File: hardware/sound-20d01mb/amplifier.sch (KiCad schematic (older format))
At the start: 30 parts

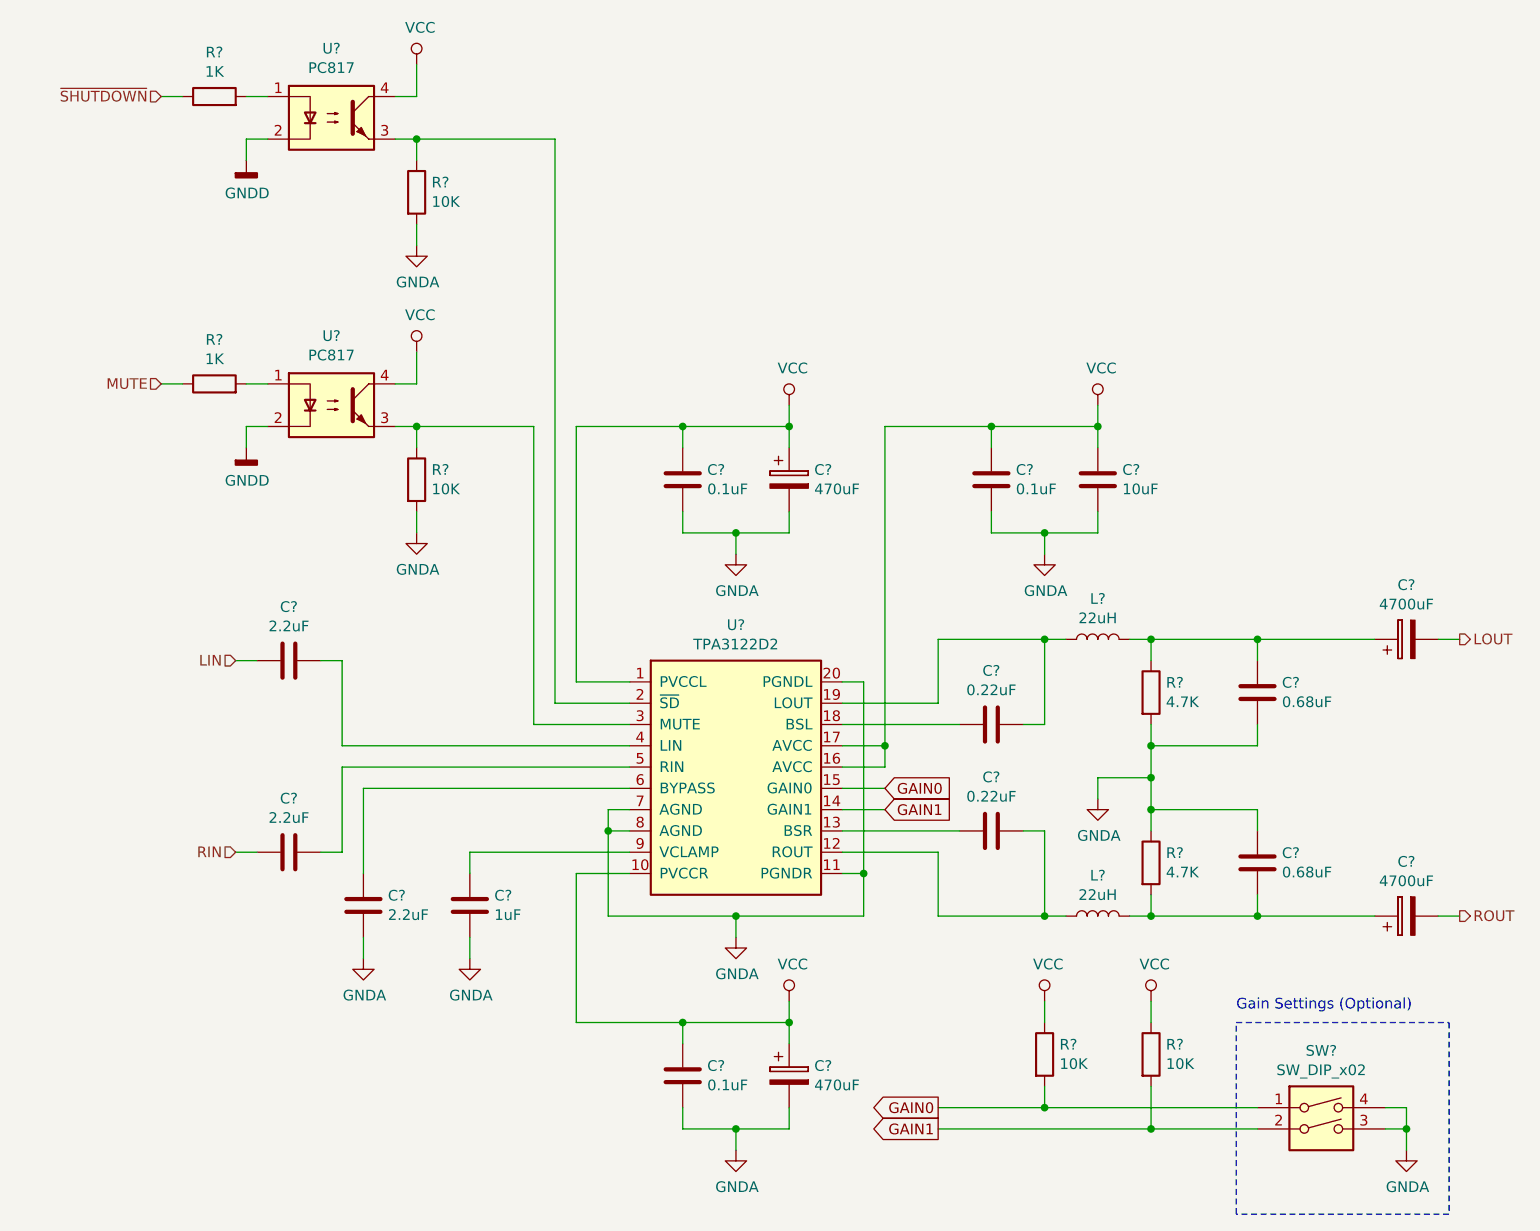
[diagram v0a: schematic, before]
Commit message: Added OSC
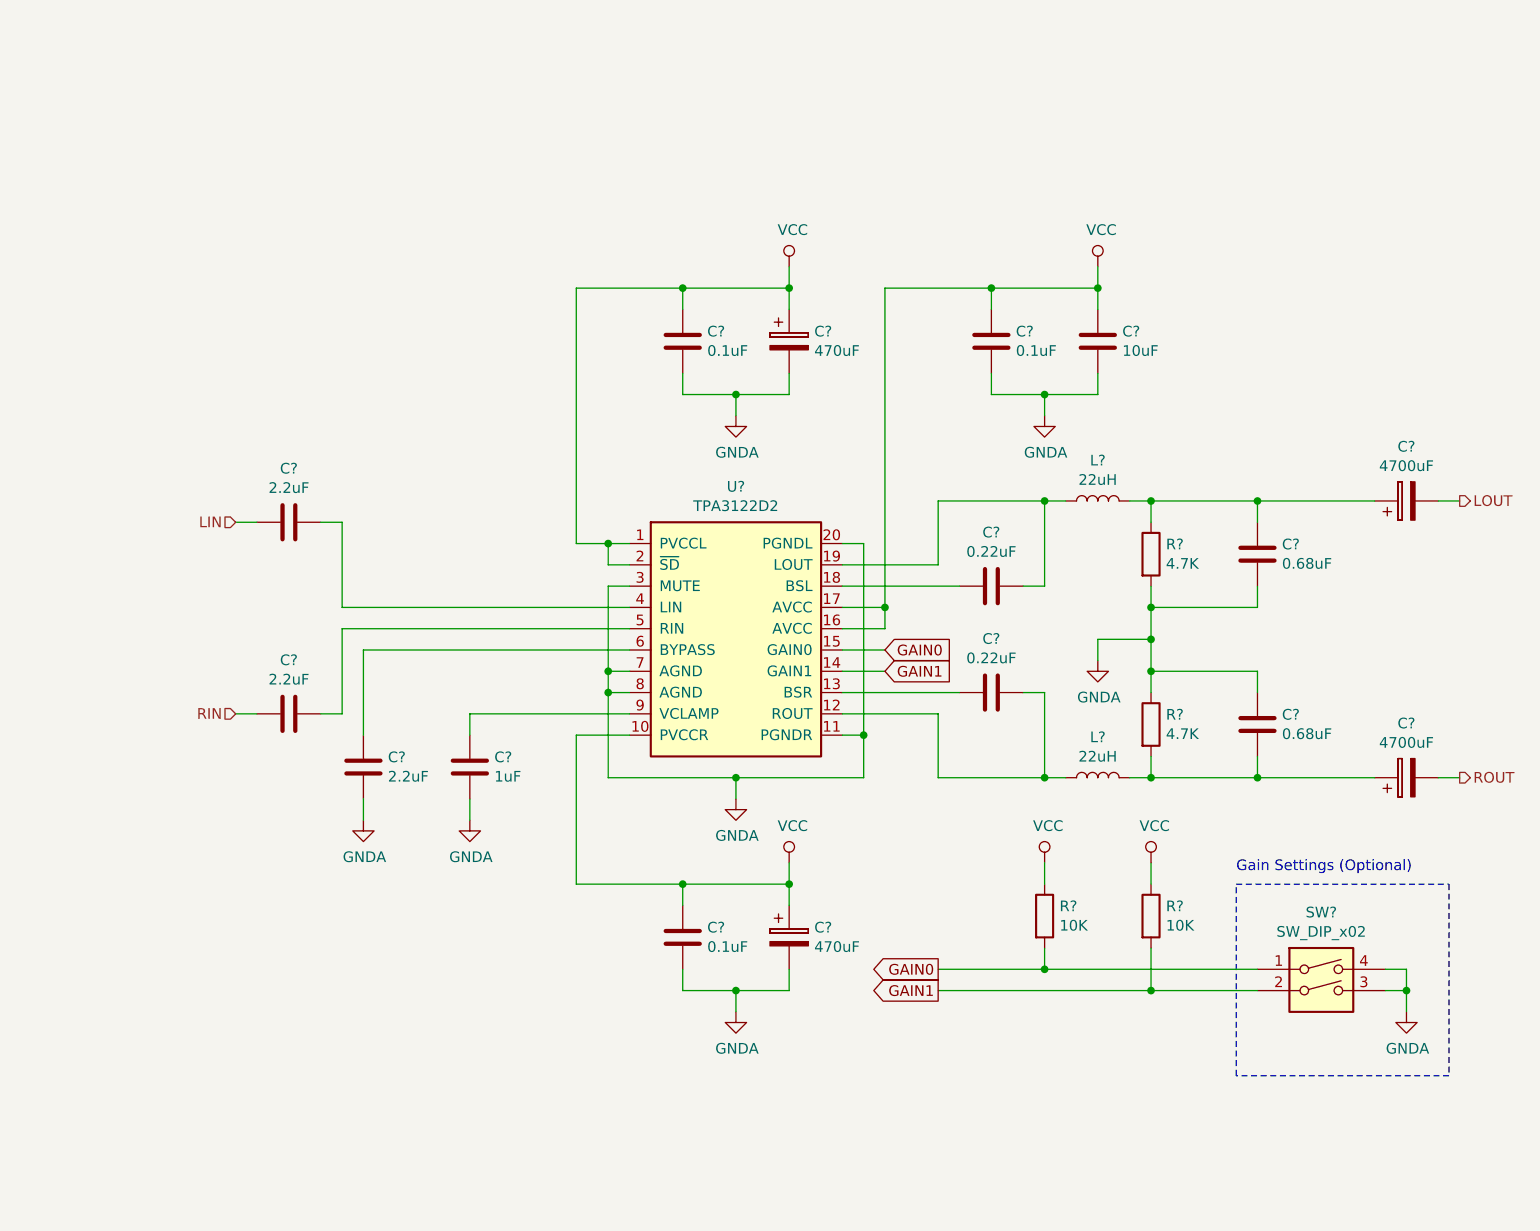
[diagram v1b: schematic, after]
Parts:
- removed R? (x2): 10K, Resistor_SMD:R_1206_3216Metric_Pad1.42x1.75mm_HandSolder, symbol Device:R
- removed R? (x2): 1K, Resistor_SMD:R_1206_3216Metric_Pad1.42x1.75mm_HandSolder, symbol Device:R
- removed U? (x2): PC817, Package_DIP:DIP-4_W7.62mm, symbol Isolator:PC817
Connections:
- net GNDA: now also U?.3 (MUTE)
- net VCC: now also U?.2 (~SD)
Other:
- moved on the sheet: C?, L?, R?, SW?, U?
